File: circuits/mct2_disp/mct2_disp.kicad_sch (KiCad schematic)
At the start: 14 parts, among them J1 20455-040E-76, J2 20455-040E-76, J3 Touch Data - I2C, J4 Touch Data - USB, J5 External Backlight Control

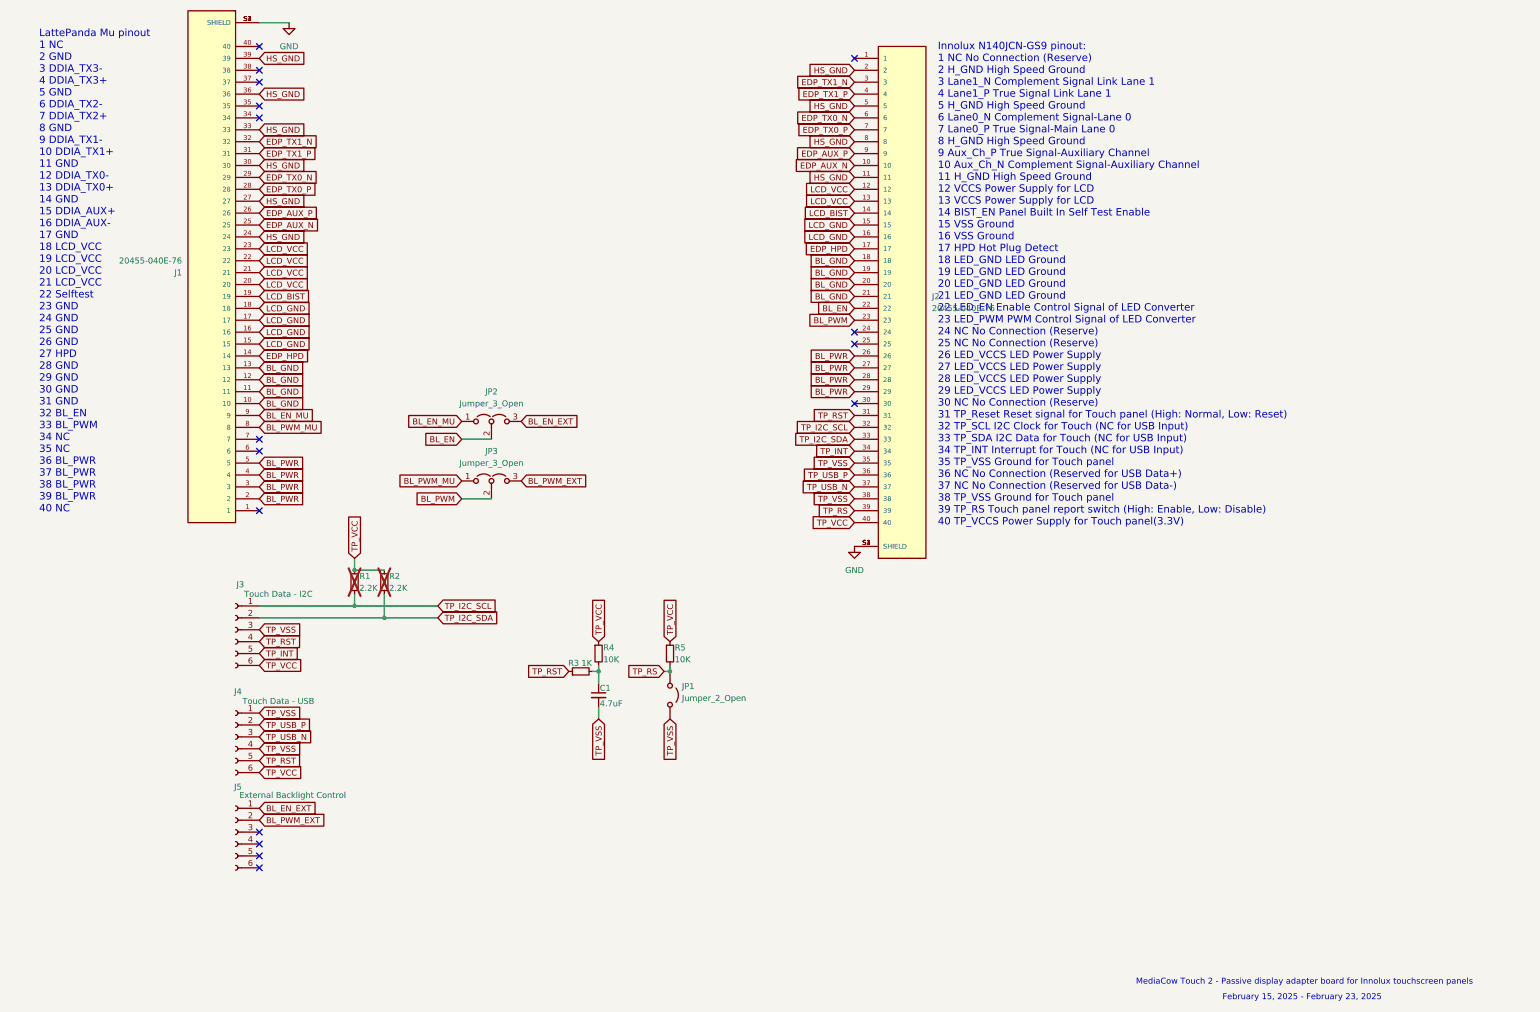
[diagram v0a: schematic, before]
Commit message: 20250224-2
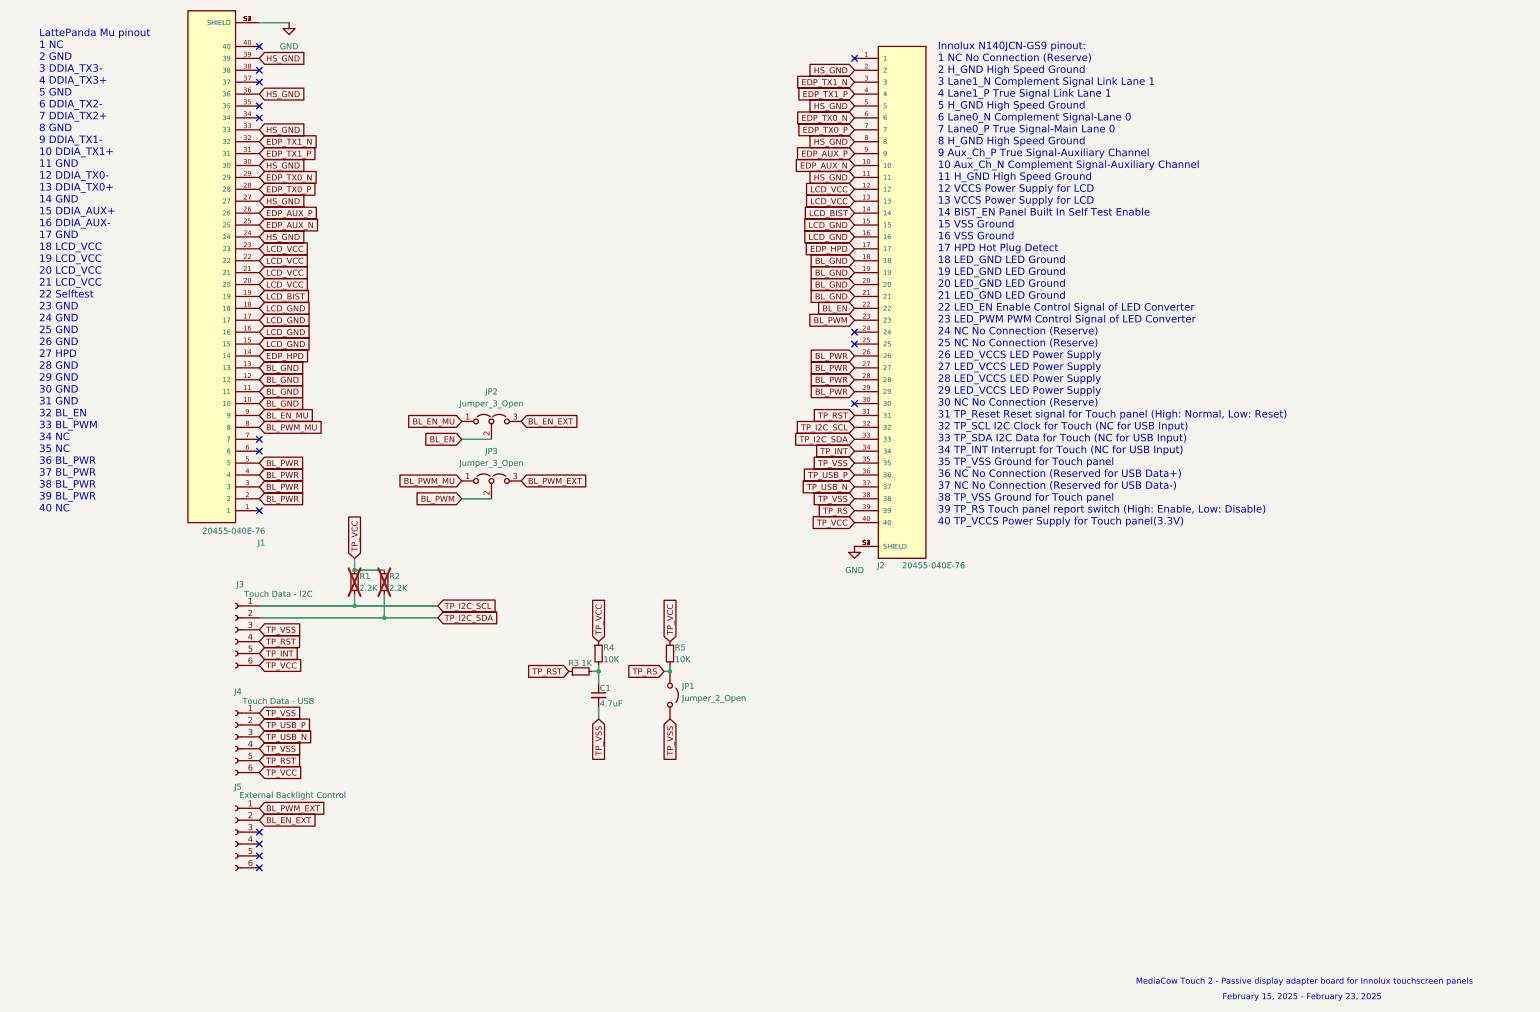
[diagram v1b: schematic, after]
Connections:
- net BL_EN_EXT: now also J5.2 (Pin_2); no longer J5.1 (Pin_1)
- net BL_PWM_EXT: now also J5.1 (Pin_1); no longer J5.2 (Pin_2)

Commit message: 20250311-1
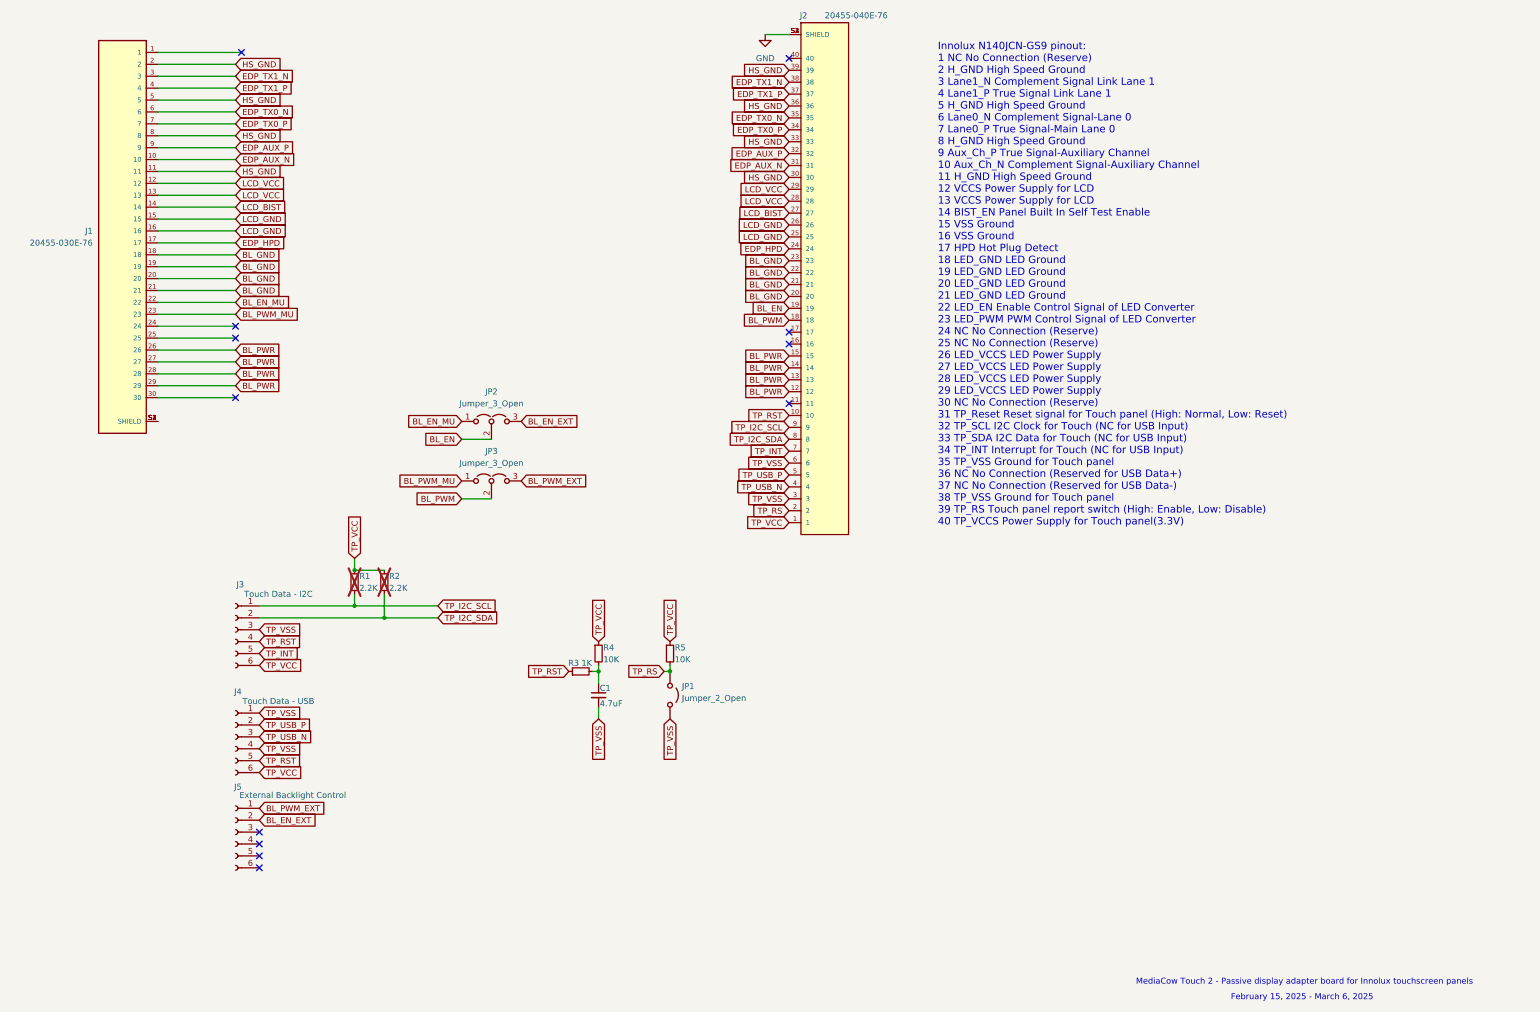
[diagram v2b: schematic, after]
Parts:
- removed J1: 20455-040E-76, MediaCow:IPEX_20455-040E-76, symbol mediacow:20455-040E-76
- added J1: 20455-030E-76, MediaCow:IPEX_20455-030E-76, symbol mediacow:20455-030E-76
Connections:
- net BL_EN: now also J2.19; no longer J2.22
- net BL_EN_MU: now also J1.22
- net BL_GND: now also J2.22, J2.23, J1.18, J1.19, J1.20, J1.21; no longer J2.18, J2.19
- net BL_PWM: now also J2.18; no longer J2.23
- net BL_PWM_MU: now also J1.23
- net BL_PWR: now also J2.12, J2.13, J2.14, J2.15, J1.26, J1.27, J1.28, J1.29; no longer J2.26, J2.27, J2.28, J2.29
- net EDP_AUX_N: now also J2.31, J1.10; no longer J2.10
- net EDP_AUX_P: now also J2.32, J1.9; no longer J2.9
- net EDP_HPD: now also J2.24, J1.17; no longer J2.17
- net EDP_TX0_N: now also J2.35, J1.6; no longer J2.6
- net EDP_TX0_P: now also J2.34, J1.7; no longer J2.7
- net EDP_TX1_N: now also J2.38, J1.3; no longer J2.3
- net EDP_TX1_P: now also J2.37, J1.4; no longer J2.4
- net HS_GND: now also J2.30, J2.33, J2.36, J2.39, J1.11, J1.2, J1.5, J1.8; no longer J2.11, J2.2, J2.5, J2.8
- net LCD_BIST: now also J2.27, J1.14; no longer J2.14
- net LCD_GND: now also J2.25, J2.26, J1.15, J1.16; no longer J2.15, J2.16
- net LCD_VCC: now also J2.28, J2.29, J1.12, J1.13; no longer J2.12, J2.13
- net TP_I2C_SCL: now also J2.9; no longer J2.32
- net TP_I2C_SDA: now also J2.8; no longer J2.33
- net TP_INT: now also J2.7; no longer J2.34
- net TP_RS: now also J2.2; no longer J2.39
- net TP_RST: now also J2.10; no longer J2.31
- net TP_USB_N: now also J2.4; no longer J2.37
- net TP_USB_P: now also J2.5; no longer J2.36
- net TP_VCC: now also J2.1; no longer J2.40
- net TP_VSS: now also J2.3, J2.6; no longer J2.35, J2.38
- new net: J1.S1 (SHIELD), J1.S2 (SHIELD), J1.S3 (SHIELD), J1.S4 (SHIELD)
- no-connect marks 16 -> 12
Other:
- note added: "February 15, 2025 - March 6, 2025"
- note removed: "February 15, 2025 - February 23, 2025"
- note removed: "LattePanda Mu pinout 1 NC 2 GND 3 DDIA_TX3- 4 DDIA_TX3+ 5 GND 6 DDIA_TX2- 7 DDIA_TX2+ 8 GND 9 DDIA_TX1- 10 DDIA_TX1+ 11 GND 12 DDIA_TX0- 13 DDIA_TX0+ 14 GND 15 DDIA_AUX+ 16 DDIA_AUX- 17 GND 18 LCD_VCC 19 LCD_VCC 20 LCD_VCC 21 LCD_VCC 22 Selftest 23 GND 24 GND 25 GND 26 GND 27 HPD 28 GND 29 GND 30 GND 31 GND 32 BL_EN 33 BL_PWM 34 NC 35 NC 36 BL_PWR 37 BL_PWR 38 BL_PWR 39 BL_PWR 40 NC"
- moved on the sheet: J2
